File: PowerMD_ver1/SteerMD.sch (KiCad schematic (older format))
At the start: 216 parts, among them P1 SWD, P10 OUT_1, P11 ENC_0, P13 ENC_1, P14 I/O_1, P15 OUT_0, P2 MOTOR_COOLING, P3 CAN, P4 CAN, P5 SERIAL, P6 I/O_0, P7 FAN, P8 BATT_IN, P9 BATT_IN, Q1 MOSFET_N, Q2 MOSFET_N, Q3 MOSFET_N, Q4 MOSFET_N, Q5 MOSFET_N, Q6 MOSFET_N, Q7 MOSFET_N, Q8 MOSFET_N, SW1 RST, SW3 SW0, SW4 SW1, U1 MAX3051, U10 ACS758, U11 POWER_ON, U12 SI8274, U13 ACS758, U14 SI8274, U15 AZ1086H, U16 LOGO, U17 AQM0802, U19 ADRESS, U2 BD9G101, U3 STM32F405RG, U4 SI8274, U5 SI8900, U6 ADC_~RST, U7 BD9G101G, U8 SI8274, U9 BD33FA1, Y1 8MHz

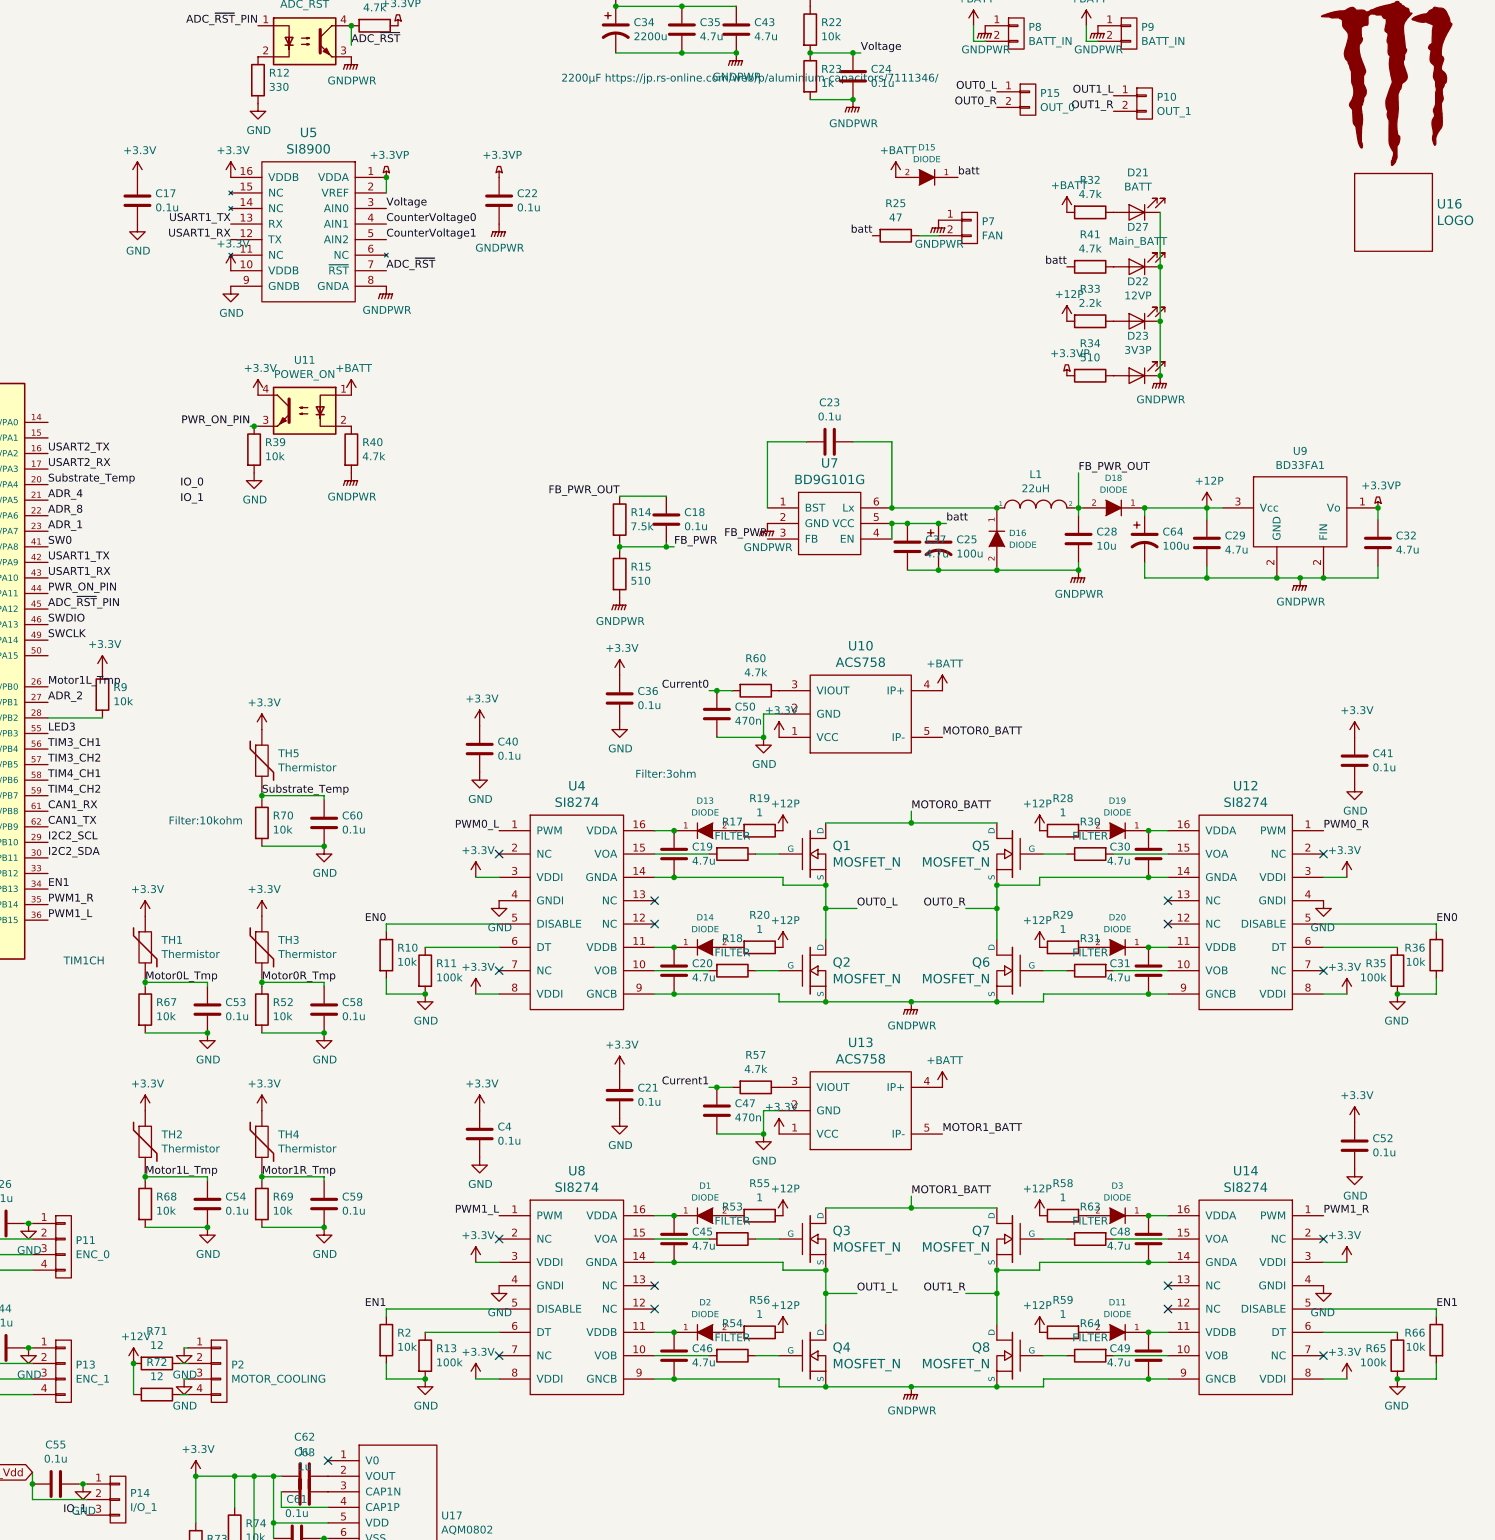
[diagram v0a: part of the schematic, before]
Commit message: 途中
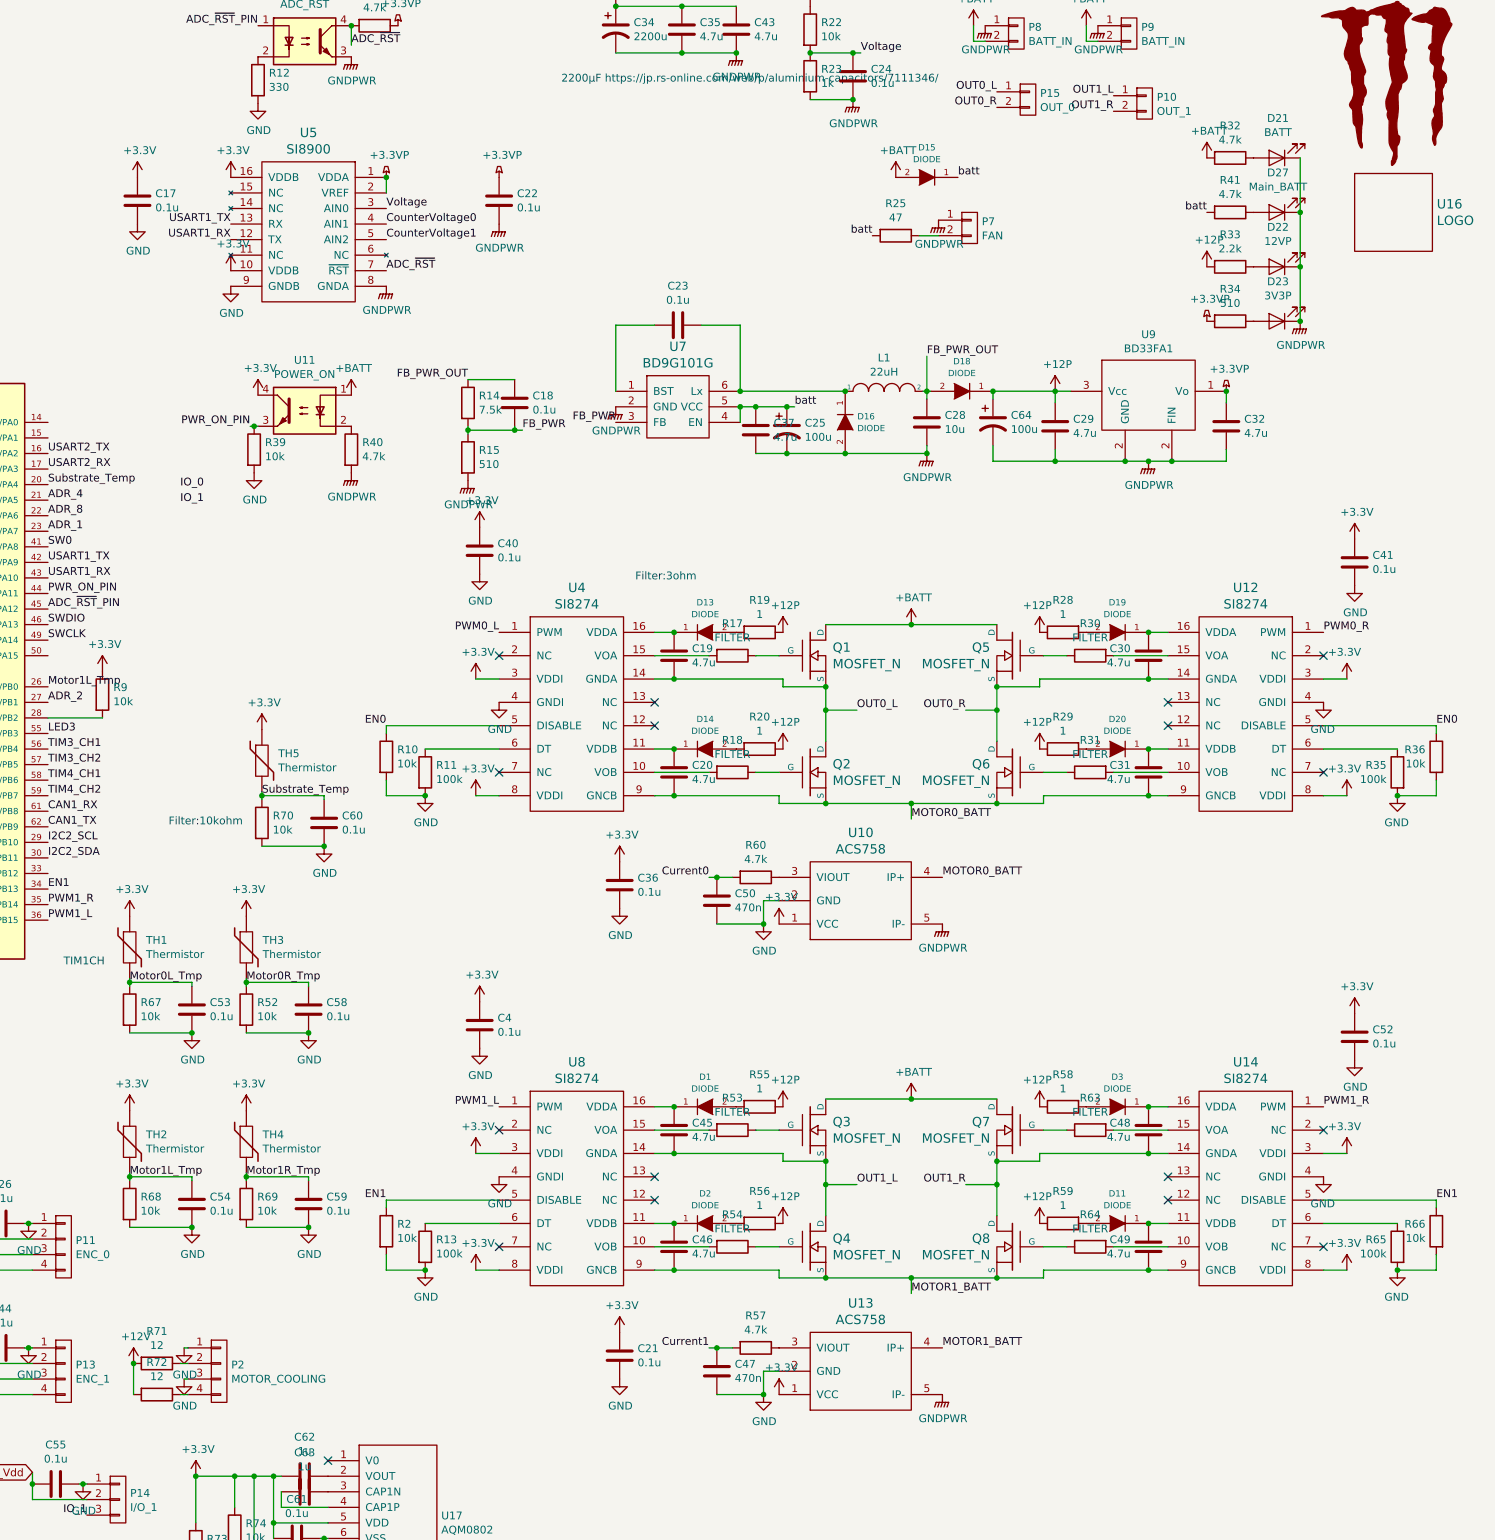
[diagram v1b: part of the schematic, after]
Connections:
- net +BATT: now also Q1.D, Q3.D, Q5.D, Q7.D; no longer U10.4 (IP+), U13.4 (IP+)
- net GNDPWR: now also U10.5 (IP-), U13.5 (IP-); no longer C20.2, C31.2, C46.2, C49.2, Q2.S, Q4.S, Q6.S, Q8.S, U12.9 (GNCB), U14.9 (GNCB), U4.9 (GNCB), U8.9 (GNCB)
- net MOTOR0_BATT: now also C20.2, C31.2, Q2.S, Q6.S, U10.4 (IP+), U12.9 (GNCB), U4.9 (GNCB); no longer Q1.D, Q5.D, U10.5 (IP-)
- net MOTOR1_BATT: now also C46.2, C49.2, Q4.S, Q8.S, U13.4 (IP+), U14.9 (GNCB), U8.9 (GNCB); no longer Q3.D, Q7.D, U13.5 (IP-)
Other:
- moved on the sheet: C18, C19, C20, C21, C23, C25, C28, C29, C30, C31, C32, C36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
